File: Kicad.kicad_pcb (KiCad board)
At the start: 4 copper layers, 54 x 54.5 mm, 35 parts, among them J1 Conn_02x07_Odd_Even, J2 Conn_01x02, J3 Conn_01x04, J4 Conn_01x02, J42 Conn_01x04, J5 Conn_01x02, J52 Conn_01x04, J6 Conn_01x03, J62 Conn_01x03, U1 STM32L021K4Tx, U2 BU33SD5WG-TR

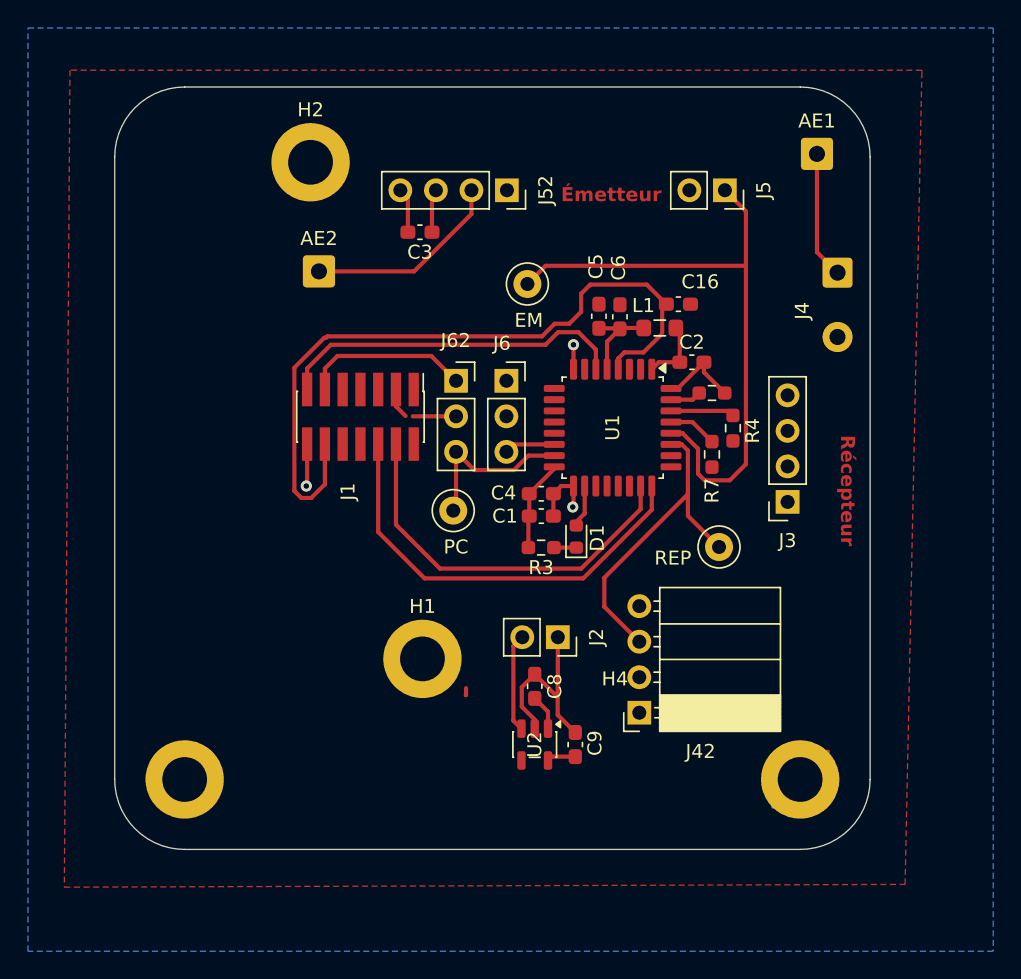
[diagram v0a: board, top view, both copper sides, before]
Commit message: test
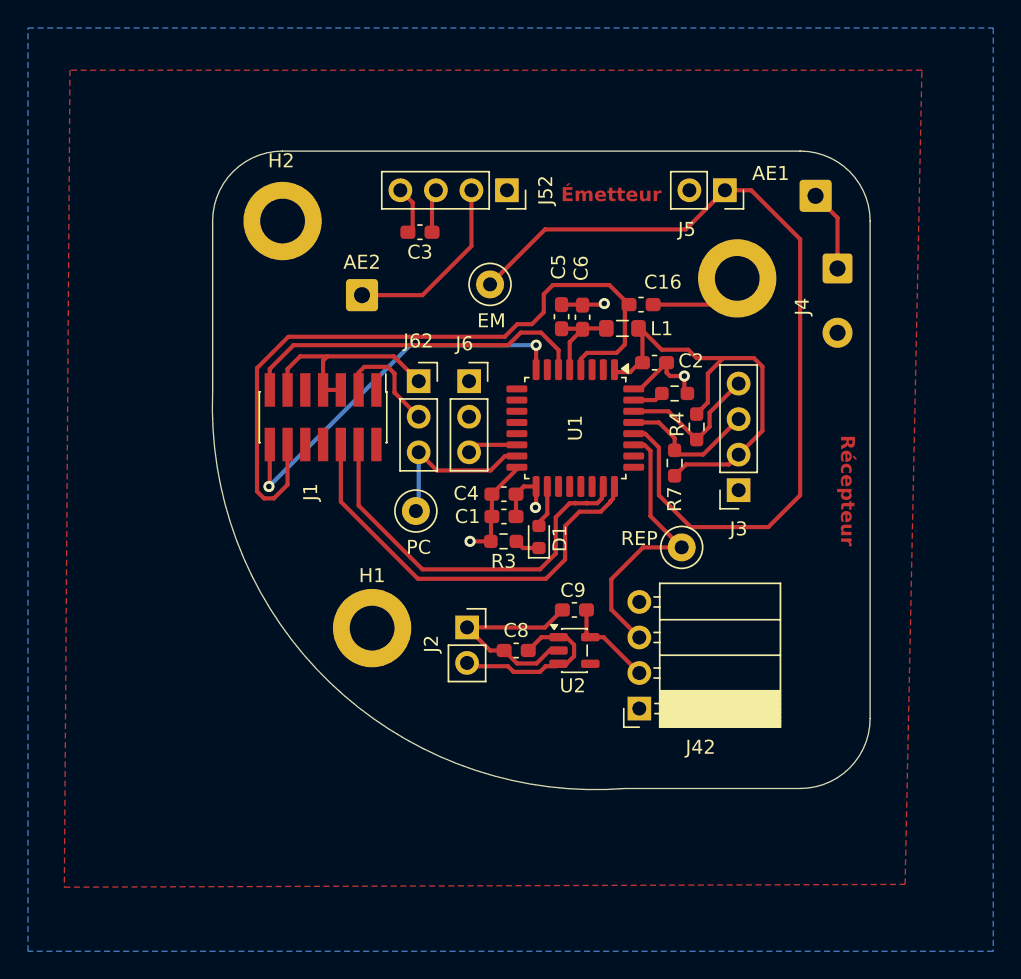
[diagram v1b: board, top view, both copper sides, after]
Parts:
- removed H4: MountingHole_Pad, MountingHole:MountingHole_3.2mm_M3_DIN965_Pad
- moved H3 53.3 mm to (172.0, 80.7)
- moved C9 9.63 mm to (160.4, 104.4), turned to 180 degrees
- moved U2 7.30 mm to (160.4, 107.3), turned to 0 degrees
- moved J2 6.53 mm to (152.7, 105.6), turned to 0 degrees
- moved H2 4.65 mm to (139.5, 76.6)
- moved H1 4.22 mm to (145.9, 105.7)
- moved J3 3.60 mm to (172.1, 95.8)
- moved AE2 3.52 mm to (145.2, 81.9)
- moved AE1 3.00 mm to (177.6, 74.8)
- moved C8 2.88 mm to (156.2, 107.3), turned to 0 degrees
- moved R7 2.74 mm to (167.5, 93.9)
- moved R3 2.72 mm to (155.3, 99.5)
- moved C1 2.67 mm to (155.3, 97.7)
- moved C4 2.67 mm to (155.3, 96.1)
- moved C5 2.67 mm to (159.4, 83.4)
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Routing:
- net GND: track 50.7 -> 202.2 mm, vias 0 -> 3
- net +3.3V: track 19.8 -> 124.4 mm
- net USART_TX: track 4.77 -> 28.1 mm
- net TX Dati: track 44.6 -> 62.3 mm
- net SCL: track 3.50 -> 9.57 mm
- net SDA: track 4.56 -> 10.6 mm
- net +5V: track 9.74 -> 13.2 mm
- net Net-(AE1-A): track 9.10 -> 5.84 mm
- net DATA_REC: track 23.3 -> 20.2 mm
- net Net-(AE2-A): track 14.3 -> 13.3 mm
- net NRST: track 51.5 -> 52.2 mm
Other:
- board size 54 x 54.5 mm -> 47 x 45.6 mm
